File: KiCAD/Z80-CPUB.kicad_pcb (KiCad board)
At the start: 2 copper layers, 99.1 x 74.9 mm, 29 parts, among them J1 SBC8080 BUS, J2 Jack-DC, M1 MountingHole_3M, M2 MountingHole_3M, M3 MountingHole_3M, M4 MountingHole_3M, U1 Z80CPU, U2 74HC14, U3 74HC04, U4 74HC32, Y1 7.3728MHz

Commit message: r1.1 最終確認
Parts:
- R5: value 4.7k -> 1k
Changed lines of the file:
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@@
       (effects (font (size 1 1) (thickness 0.15)))
     )
-    (fp_text value D (at 5.08 2.41) (layer F.Fab)
-      (effects (font (size 1 1) (thickness 0.15)))
-    )
-    (fp_text user %R (at 5.08 -2.54) (layer F.Fab)
+    (fp_text value D (at 5.376 0.174) (layer F.Fab)
+      (effects (font (size 1 1) (thickness 0.15)))
+    )
+    (fp_text user %R (at 5.376 2.206) (layer F.Fab)
       (effects (font (size 1 1) (thickness 0.15)))
     )
@@
       (effects (font (size 1 1) (thickness 0.15)))
     )
-    (fp_text value 3.3k (at 3.81 2.54) (layer F.Fab)
+    (fp_text value 3.3k (at 4.064 0) (layer F.Fab)
       (effects (font (size 1 1) (thickness 0.15)))
     )
@@
       (effects (font (size 1 1) (thickness 0.15)))
     )
-    (fp_text value 2.2k (at 3.81 2.31) (layer F.Fab)
+    (fp_text value 2.2k (at 4.086 -0.176) (layer F.Fab)
       (effects (font (size 1 1) (thickness 0.15)))
     )
@@
       (effects (font (size 1 1) (thickness 0.15)))
     )
-    (fp_text value 1k (at 3.81 -1.905 180) (layer F.Fab)
+    (fp_text value 1k (at 4.064 0 180) (layer F.Fab)
       (effects (font (size 1 1) (thickness 0.15)))
     )
@@
       (effects (font (size 1 1) (thickness 0.15)))
     )
-    (fp_text value 1M (at 3.81 -1.905 180) (layer F.Fab)
+    (fp_text value 1M (at 4.064 0 180) (layer F.Fab)
       (effects (font (size 1 1) (thickness 0.15)))
     )
@@
       (effects (font (size 1 1) (thickness 0.15)))
     )
-    (fp_text value SW (at 2.11 3.14) (layer F.Fab)
+    (fp_text value SW (at -2.54 0) (layer F.Fab)
       (effects (font (size 1 1) (thickness 0.15)))
     )
@@
       (effects (font (size 1 1) (thickness 0.15)))
     )
-    (fp_text value 4.7k (at 3.81 2.31 180) (layer F.Fab)
-      (effects (font (size 1 1) (thickness 0.15)))
-    )
+    (fp_text value 1k (at 3.81 0.018 180) (layer F.Fab)
+      (effects (font (size 1 1) (thickness 0.15)))
+    )

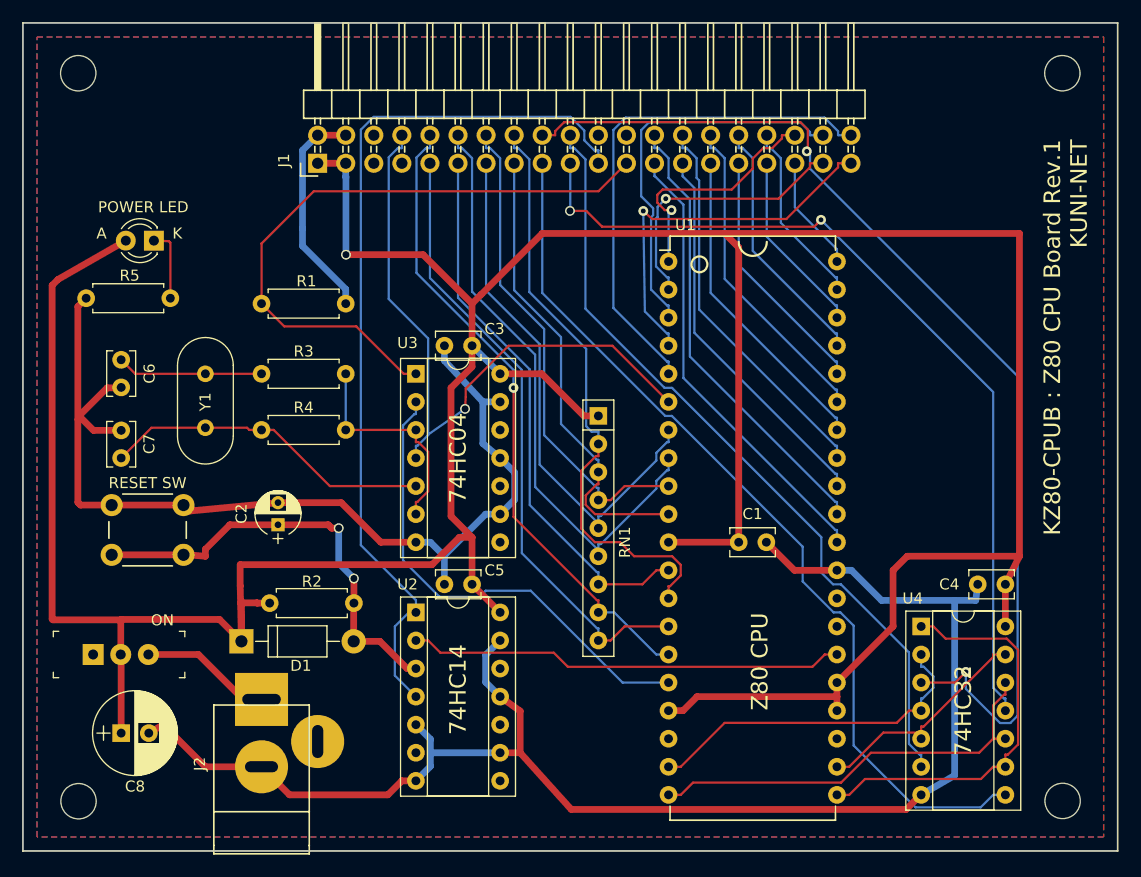
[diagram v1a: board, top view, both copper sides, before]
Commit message: REV2 回路図、製造データ出力
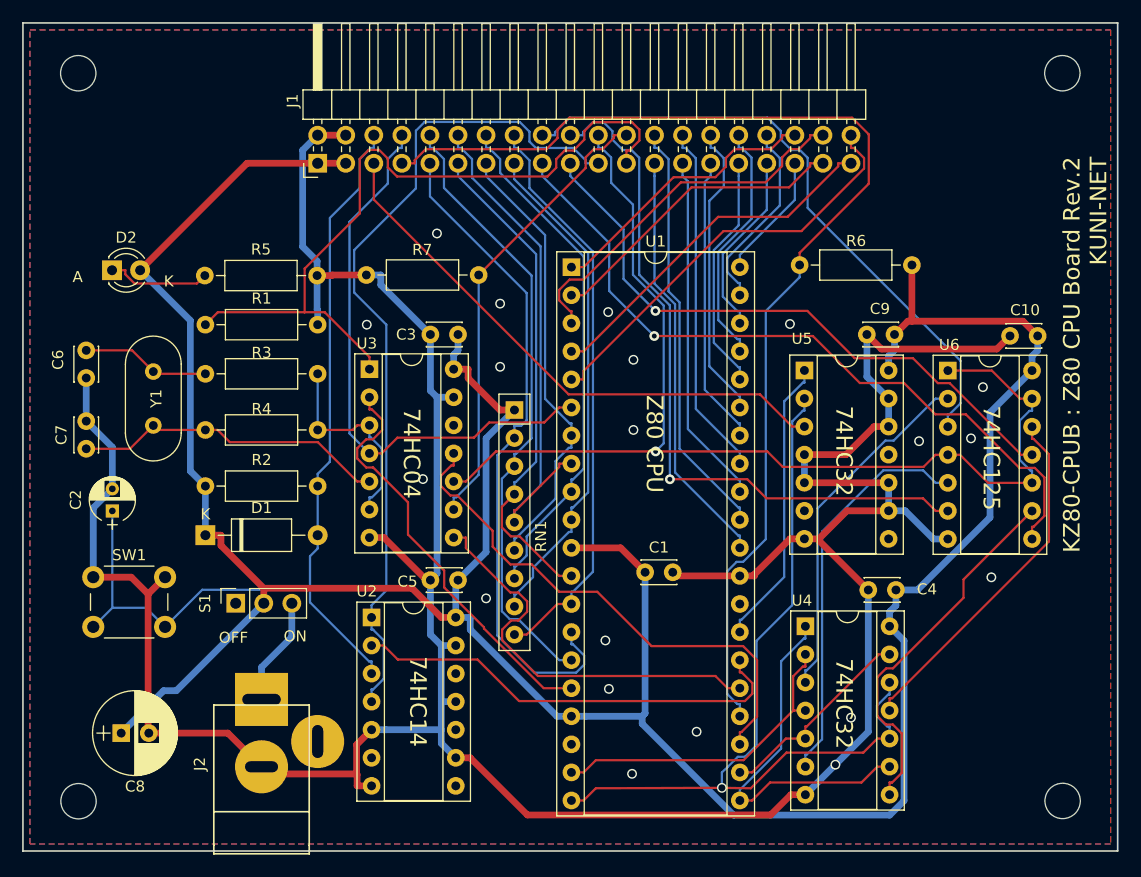
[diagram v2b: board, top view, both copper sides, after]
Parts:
- removed ON: SW, digikey-footprints:Switch_Slide_11.6x4mm_EG1218
- removed POWER LED: LED, LEDs:LED_D3.0mm
- removed RESET SW: RESET SW, Buttons_Switches_THT:SW_PUSH_6mm
- added C10: 0.1u, Capacitor_THT:C_Disc_D3.0mm_W2.0mm_P2.50mm, F.Cu at (156.6, 85.5)
- added C9: 0.1u, Capacitor_THT:C_Disc_D3.0mm_W2.0mm_P2.50mm, F.Cu at (143.6, 85.3)
- added D2: LED, LED_THT:LED_D3.0mm, F.Cu at (72.8, 79.5)
- added R6: 4.7k, Resistor_THT:R_Axial_DIN0207_L6.3mm_D2.5mm_P10.16mm_Horizontal, F.Cu at (145.2, 79.1)
- added R7: 4.7k, Resistor_THT:R_Axial_DIN0207_L6.3mm_D2.5mm_P10.16mm_Horizontal, F.Cu at (106.0, 80.0)
- added S1: SW, Connector_PinSocket_2.54mm:PinSocket_1x03_P2.54mm_Vertical, F.Cu at (84.0, 109.7)
- added SW1: RESET SW, Button_Switch_THT:SW_PUSH_6mm_H4.3mm, F.Cu at (71.1, 107.3)
- added U5: 74HC32, Package_DIP:DIP-14_W7.62mm_Socket, F.Cu at (135.5, 88.6)
- added U6: 74HC125, Package_DIP:DIP-14_W7.62mm_Socket, F.Cu at (148.5, 88.6)
- C1, C3, C4, C5, C6, C7: footprint Capacitors_THT:C_Rect_L4.0mm_W2.5mm_P2.50mm -> Capacitor_THT:C_Disc_D3.0mm_W2.0mm_P2.50mm
- D1: footprint Diodes_THT:D_DO-41_SOD81_P10.16mm_Horizontal -> Diode_THT:D_A-405_P10.16mm_Horizontal
- J1: footprint Pin_Headers:Pin_Header_Angled_2x20 -> Connector_PinHeader_2.54mm:PinHeader_2x20_P2.54mm_Horizontal
- M1, M2, M3, M4: footprint Mounting_Holes:MountingHole_3.2mm_M3 -> MountingHole:MountingHole_3.2mm_M3
- R1: value 3.3k -> 4.7k; footprint Resistors_THT:R_Axial_DIN0207_L6.3mm_D2.5mm_P7.62mm_Horizontal -> Resistor_THT:R_Axial_DIN0207_L6.3mm_D2.5mm_P10.16mm_Horizontal
- R2: value 2.2k -> 4.7k; footprint Resistors_THT:R_Axial_DIN0207_L6.3mm_D2.5mm_P7.62mm_Horizontal -> Resistor_THT:R_Axial_DIN0207_L6.3mm_D2.5mm_P10.16mm_Horizontal
- R3, R4, R5: footprint Resistors_THT:R_Axial_DIN0207_L6.3mm_D2.5mm_P7.62mm_Horizontal -> Resistor_THT:R_Axial_DIN0207_L6.3mm_D2.5mm_P10.16mm_Horizontal
- RN1: value R_Network08 -> 10k
- U1: footprint Housings_DIP:DIP-40_W15.24mm -> Package_DIP:DIP-40_W15.24mm_Socket
- U2, U3, U4: footprint Housings_DIP:DIP-14_W7.62mm_Socket -> Package_DIP:DIP-14_W7.62mm_Socket
- Y1: footprint Crystals:Crystal_HC49-4H_Vertical -> Crystal:Crystal_HC49-U_Vertical
- moved C2 15.0 mm to (72.9, 101.3)
- moved R2 12.1 mm to (81.3, 99.1)
- moved U4 10.5 mm to (135.6, 111.7)
- moved D1 10.1 mm to (81.3, 103.5)
- moved C4 9.92 mm to (143.8, 108.5)
- moved C1 8.90 mm to (121.1, 106.9)
- moved U1 8.80 mm to (114.4, 79.2)
- moved RN1 7.61 mm to (109.2, 92.2)
- moved R1 5.43 mm to (81.3, 84.5)
- moved Y1 4.72 mm to (76.6, 88.7)
- moved U3 4.22 mm to (96.1, 88.5)
- moved U2 4.04 mm to (96.3, 110.9)
- moved R5 3.73 mm to (81.2, 80.0), turned to 0 degrees
- moved C6 3.27 mm to (70.5, 86.8)
- moved C7 3.27 mm to (70.5, 95.7)
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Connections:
- C2 pad 1: Net-(C2-Pad1) -> ~RESIN
- D1 pad 2: Net-(C2-Pad1) -> ~RESIN
- J1 pad 22: Net-(J1-Pad22) -> HLDA
- J1 pad 24: Net-(J1-Pad24) -> HOLD
- J1 pad 5: Net-(J1-Pad5) -> ~INTA
- J1 pad 6: Net-(J1-Pad6) -> ~RESIN
- J1 pad 7: Net-(J1-Pad7) -> RDYIN
- R2 pad 2: Net-(C2-Pad1) -> ~RESIN
- RN1 pad 2: D7 -> D0
- RN1 pad 3: D6 -> D1
- RN1 pad 4: D5 -> D2
- RN1 pad 5: D4 -> D3
- RN1 pad 6: D3 -> D4
- RN1 pad 7: D2 -> D5
- RN1 pad 8: D1 -> D6
- RN1 pad 9: D0 -> D7
- U1 pad 24: VCC -> RDYIN
- U1 pad 25: VCC -> Net-(U1-Pad25)
- U2 pad 3: Net-(C2-Pad1) -> ~RESIN
- U3 pad 10: Net-(U3-Pad10) -> HLDA
- U3 pad 11: GND -> Net-(U1-Pad23)
- U3 pad 8: Net-(U3-Pad8) -> Net-(U1-Pad25)
- U3 pad 9: GND -> HOLD
- U4 pad 11: ~IOWR -> Net-(U4-Pad11)
- U4 pad 3: ~MEMRD -> Net-(U4-Pad3)
- U4 pad 6: ~MEMWR -> Net-(U4-Pad6)
- U4 pad 8: ~IORD -> Net-(U4-Pad8)
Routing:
- net HLDA: track 0.00 -> 104.5 mm, vias 0 -> 1
- net RDYIN: track 0.00 -> 104.1 mm
- net ~RESIN: track 0.00 -> 84.9 mm
- net VCC: track 335.9 -> 268.4 mm, vias 1 -> 0
- net ~INTA: track 0.00 -> 50.8 mm
- net Net-(U1-Pad23): track 0.00 -> 47.9 mm
- net GND: track 247.7 -> 293.5 mm, vias 0 -> 20
- net HOLD: track 0.00 -> 41.6 mm
- net ~MEMRD: track 98.2 -> 57.4 mm, vias 2 -> 0
- net Net-(C2-Pad1): track 39.7 -> 0.00 mm, vias 2 -> 0
- net /~IOREQ: track 38.2 -> 76.1 mm, vias 0 -> 1
- net Net-(U1-Pad25): track 0.00 -> 37.7 mm
- net Net-(U4-Pad6): track 0.00 -> 36.1 mm
- net Net-(U4-Pad8): track 0.00 -> 33.7 mm
- net Net-(U4-Pad11): track 0.00 -> 32.5 mm
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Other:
- board text added: "74HC125"
- board text added: "KZ80-CPUB : Z80 CPU Board Rev.2 KUNI-NET"
- board text added: "OFF"
- board text added: "ON"
- board text removed: "KZ80-CPUB : Z80 CPU Board Rev.1 KUNI-NET"
